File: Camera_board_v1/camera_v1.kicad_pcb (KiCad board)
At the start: 2 copper layers, 21.4 x 36.6 mm, 27 parts, among them J1 Conn_01x01, J10 I2C1 Breakout, J7 FC Connector, J8 I2C1 Breakout, J9 I2C1 Breakout, U2 TLV74315, U3 TLV74328, X1 CAMERA_OV2640

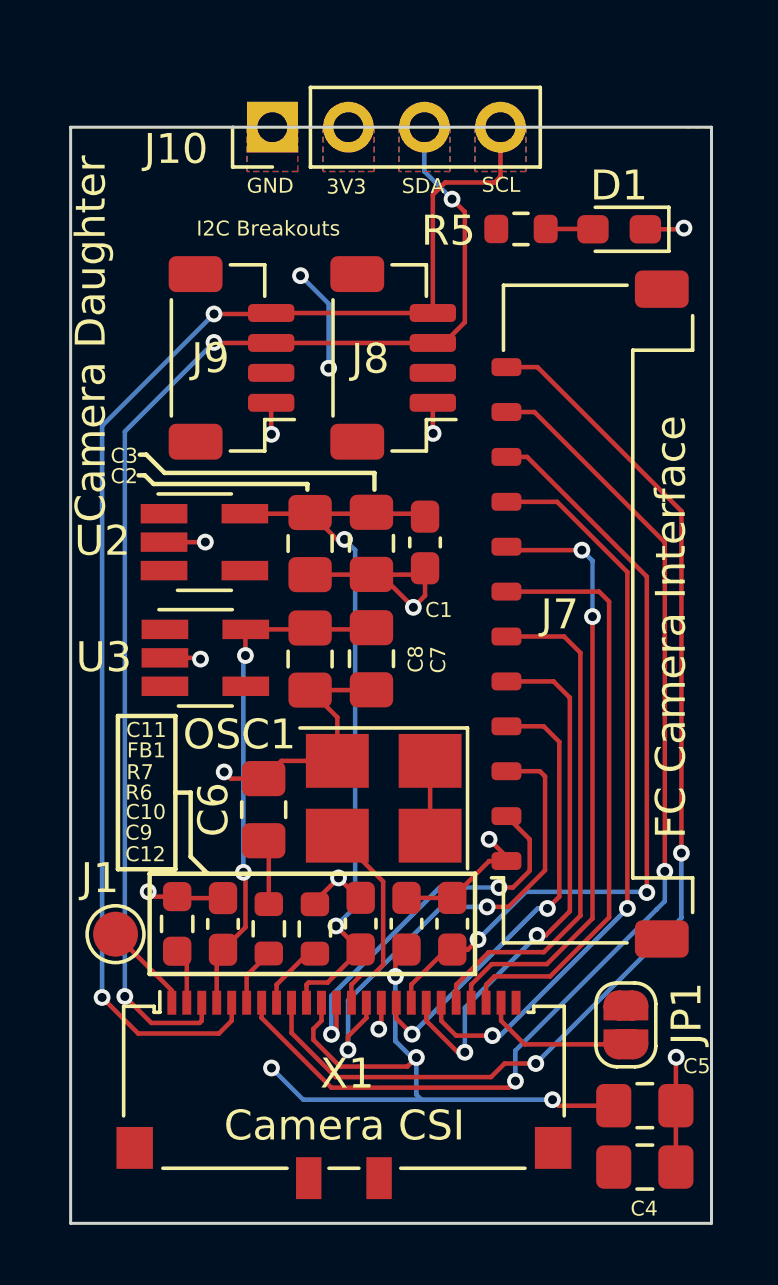
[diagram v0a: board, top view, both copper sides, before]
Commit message: Big Update of In Dev Boards
Mid Term update for all the boards being developed for use by the Irvington Team on Pleiades - Orpheus
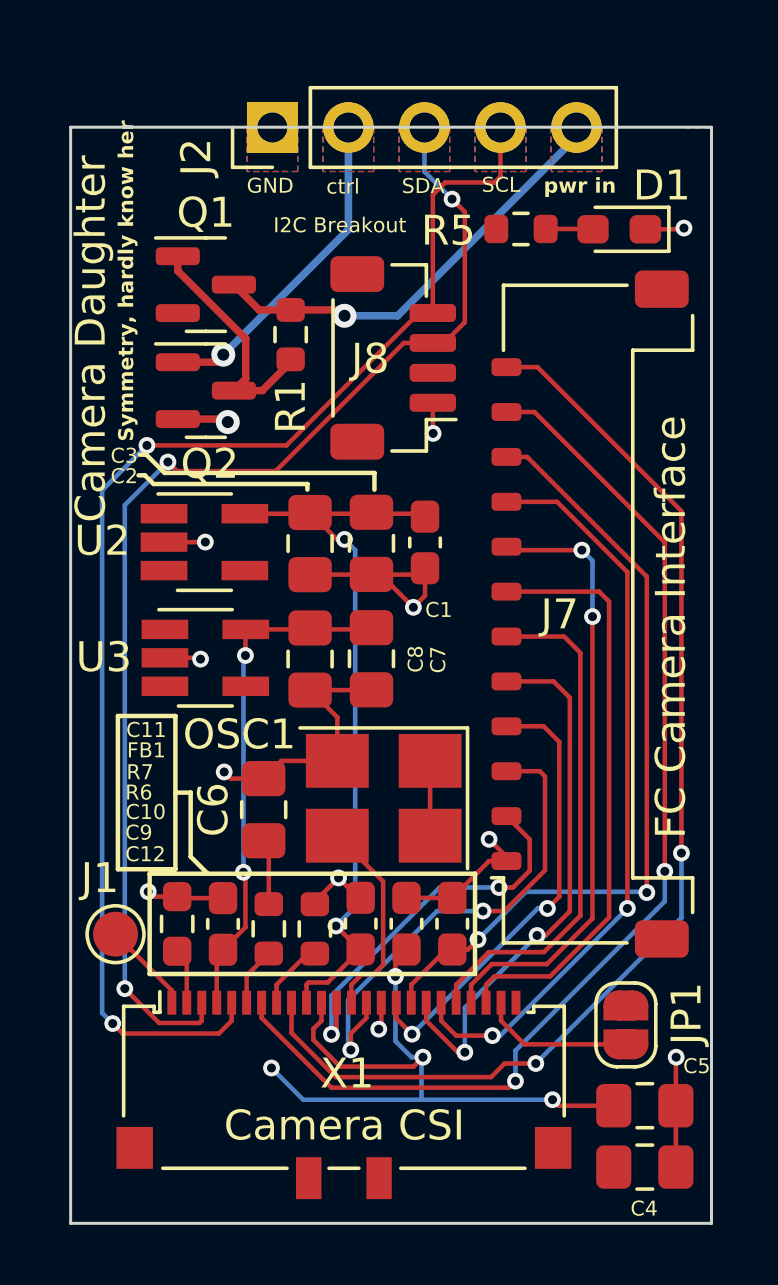
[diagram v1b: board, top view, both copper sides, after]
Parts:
- removed J10: I2C1 Breakout, Connector_PinHeader_2.54mm:PinHeader_1x04_P2.54mm_Vertical
- removed J9: I2C1 Breakout, Connector_JST:JST_SH_BM04B-SRSS-TB_1x04-1MP_P1.00mm_Vertical
- added G***: LOGO, LOGO, B.Cu at (157.5, 126.4)
- added J2: Conn_01x05, Connector_PinHeader_2.54mm:PinHeader_1x05_P2.54mm_Vertical, F.Cu at (153.7, 105.7)
- added Q1: BSS83P, Package_TO_SOT_SMD:SOT-23, F.Cu at (151.5, 110.9)
- added Q2: BSS138, Package_TO_SOT_SMD:SOT-23, F.Cu at (151.5, 114.5)
- added R1: 10K, Resistor_SMD:R_0603_1608Metric, F.Cu at (154.3, 112.6)
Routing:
- net pwr_in: track 0.00 -> 14.4 mm, vias 0 -> 1
- net pwr_ctrl: track 0.00 -> 10.6 mm, vias 0 -> 1
- net Net-(Q1-G): track 0.00 -> 7.98 mm
- net +3V3: track 31.0 -> 28.0 mm, vias 6 -> 4
- net SDA1: track 42.2 -> 40.8 mm
- net SCL1: track 45.2 -> 44.3 mm
- net GND: track 36.4 -> 37.0 mm
- added copper zone on B.Cu, net pwr_ctrl
- added copper zone on F.Cu, net pwr_ctrl
- added copper zone on B.Cu, net pwr_in
- added copper zone on F.Cu, net pwr_in
- removed copper zone on B.Cu, net +3V3
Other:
- board text added: "I2C Breakout"
- board text added: "Symmetry, hardly know her"
- board text added: "ctrl"
- board text added: "pwr in"
- board text removed: "3V3"
- board text removed: "I2C Breakouts"
